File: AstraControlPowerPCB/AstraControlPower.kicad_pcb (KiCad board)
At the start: 4 copper layers, 40 x 60 mm, 1 part, among them CN1 WJ124_5P

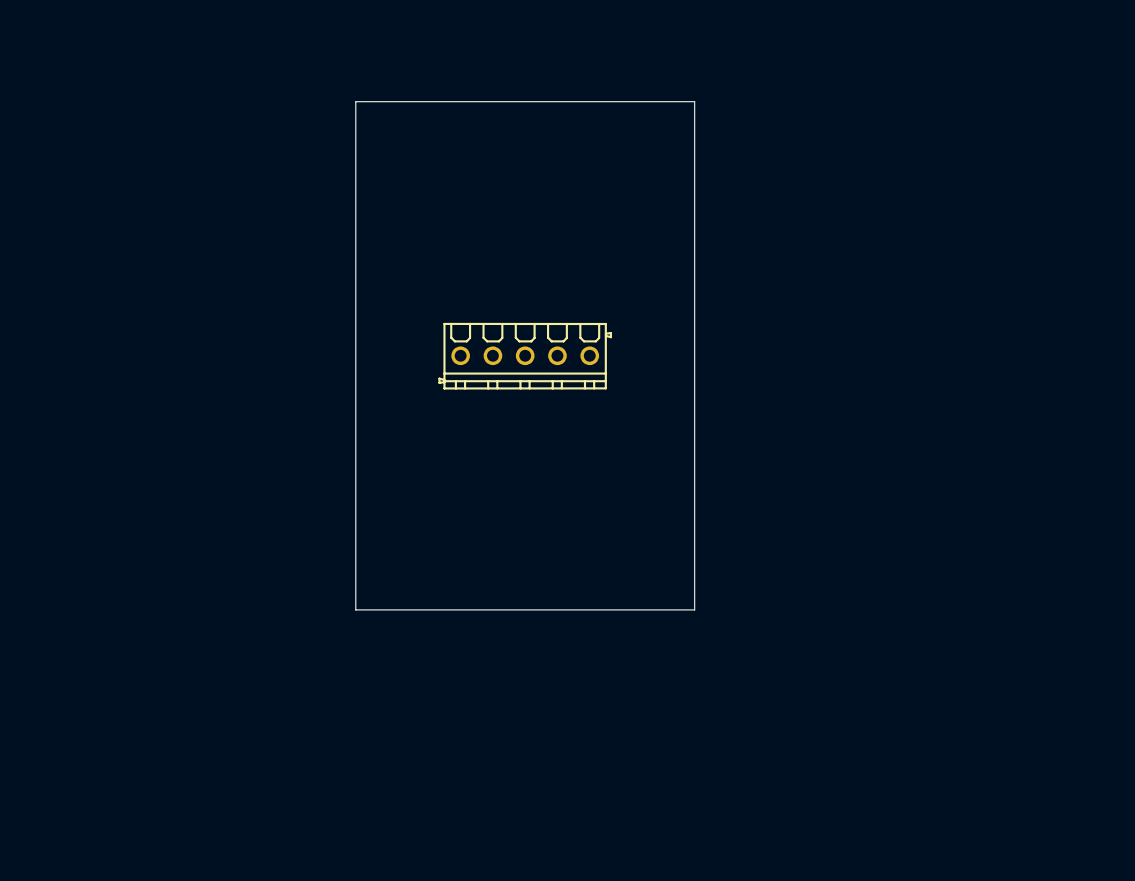
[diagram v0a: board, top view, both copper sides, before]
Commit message: Finished layout
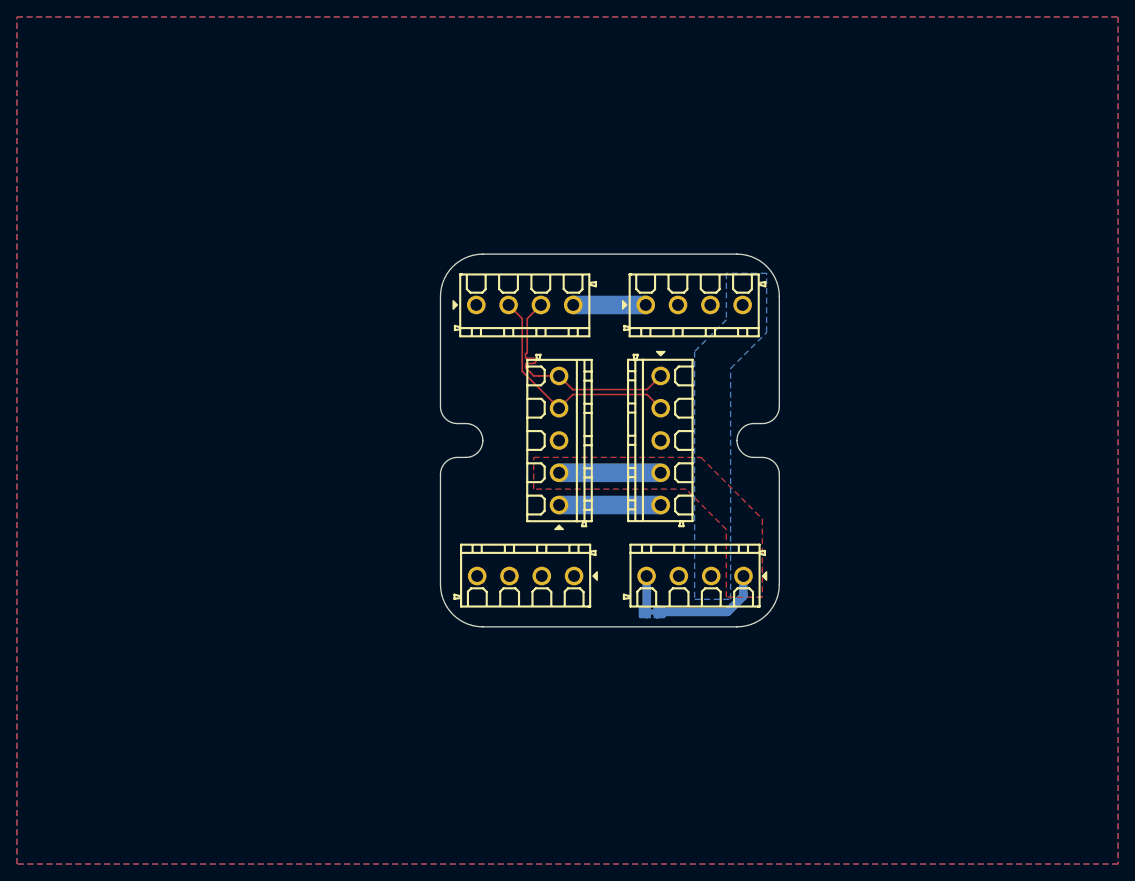
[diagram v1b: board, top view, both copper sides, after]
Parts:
- added CN2: WJ124_5P, LiveAstra:CN_SCREW_TERMINAL_WJ124_4P-P3.81_KF124-4P, F.Cu at (170.0, 126.0)
- added CN3: WJ124_5P, LiveAstra:CN_SCREW_TERMINAL_WJ124_4P-P3.81_KF124-4P, F.Cu at (170.0, 94.0)
- added CN4: WJ124_5P, LiveAstra:CN_SCREW_TERMINAL_WJ124_4P-P3.81_KF124-4P, F.Cu at (150.0, 94.0)
- added CN5: WJ124_5P, LiveAstra:CN_SCREW_TERMINAL_WJ124_4P-P3.81_KF124-4P, F.Cu at (150.0, 126.0)
- added CN6: WJ124_5P, LiveAstra:CN_SCREW_TERMINAL_WJ124_5P-P3.81_KF124-5P, F.Cu at (166.0, 110.0)
- added JP1: JP_SolderJumper_2_Bridged, Jumper:SolderJumper-2_P1.3mm_Bridged_RoundedPad1.0x1.5mm, B.Cu at (165.0, 130.2)
- CN1: footprint LiveAstra:CN_SCREW_TERMINAL_WJ124_5P-P3.81_KF124-3.81-5P -> LiveAstra:CN_SCREW_TERMINAL_WJ124_5P-P3.81_KF124-5P
- moved CN1 10.8 mm to (154.0, 110.0), turned to 90 degrees
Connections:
- CN1 pad 1: unconnected-(CN1-Pin_1-Pad1) -> /Block Diagram/5V
- CN1 pad 2: unconnected-(CN1-Pin_2-Pad2) -> /Block Diagram/VIN
- CN1 pad 3: unconnected-(CN1-Pin_3-Pad3) -> GND
- CN1 pad 4: unconnected-(CN1-Pin_4-Pad4) -> /Block Diagram/RS485+
- CN1 pad 5: unconnected-(CN1-Pin_5-Pad5) -> /Block Diagram/RS485-
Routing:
- net /Block Diagram/RS485+: track 0.00 -> 28.0 mm
- net /Block Diagram/RS485-: track 0.00 -> 28.0 mm
- net /Block Diagram/VIN: track 0.00 -> 24.9 mm
- net /Block Diagram/5V: track 0.00 -> 20.6 mm
- net /Block Diagram/LED: track 0.00 -> 4.51 mm
- added copper zone on In2.Cu, net /Block Diagram/5V
- added copper zone on F.Cu, net /Block Diagram/VIN
- added copper zone on B.Cu, net /Block Diagram/VIN_SW
- added copper zone on B.Cu, net GND
- added copper zone on F.Cu, net GND
- added copper zone on In1.Cu, net GND
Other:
- board size 40 x 60 mm -> 40 x 44 mm
